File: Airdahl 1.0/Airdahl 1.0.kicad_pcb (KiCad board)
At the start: 2 copper layers, 57.6 x 39.5 mm, 94 parts, among them J1 Conn_01x04, J2 DF40C-34DS-0.4V_58_, J3 DF40C-34DS-0.4V_58_, J4 USB_C_Receptacle_USB2.0_16P, J7 CONUFL001-SMD-T, J9 104031-0811, SW1 SW_SPST, SW2 SW_SPST, U1 STM32F446RETx, U2 MCP2200-I-MQ, U4 BNO085, U5 BMP581, U6 RFM95W-915S2, U7 NCP1117-3.3_SOT223, Y1 ABM3B-8.000MHZ-12-D1X-T, Y2 ABS25-32.768KHZ-6-T, Y3 12MHz

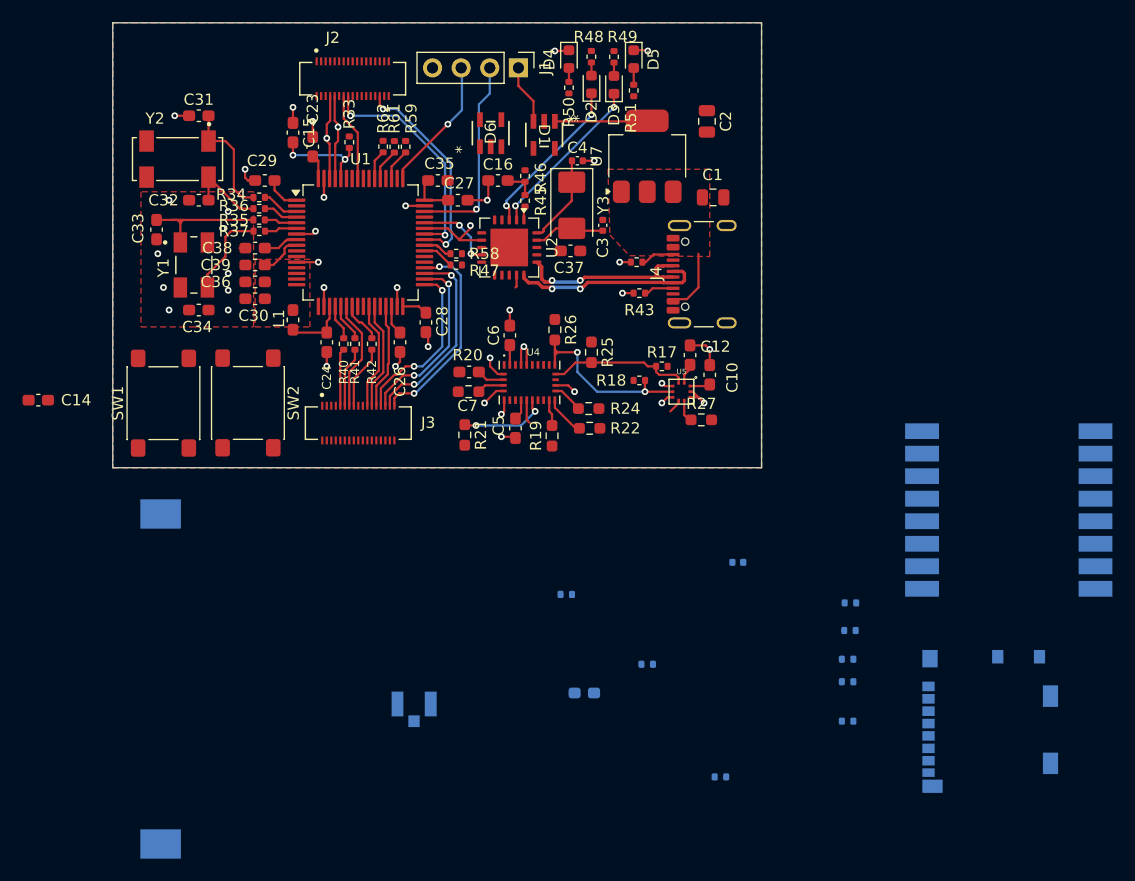
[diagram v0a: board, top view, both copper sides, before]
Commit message: dumping many layout changes
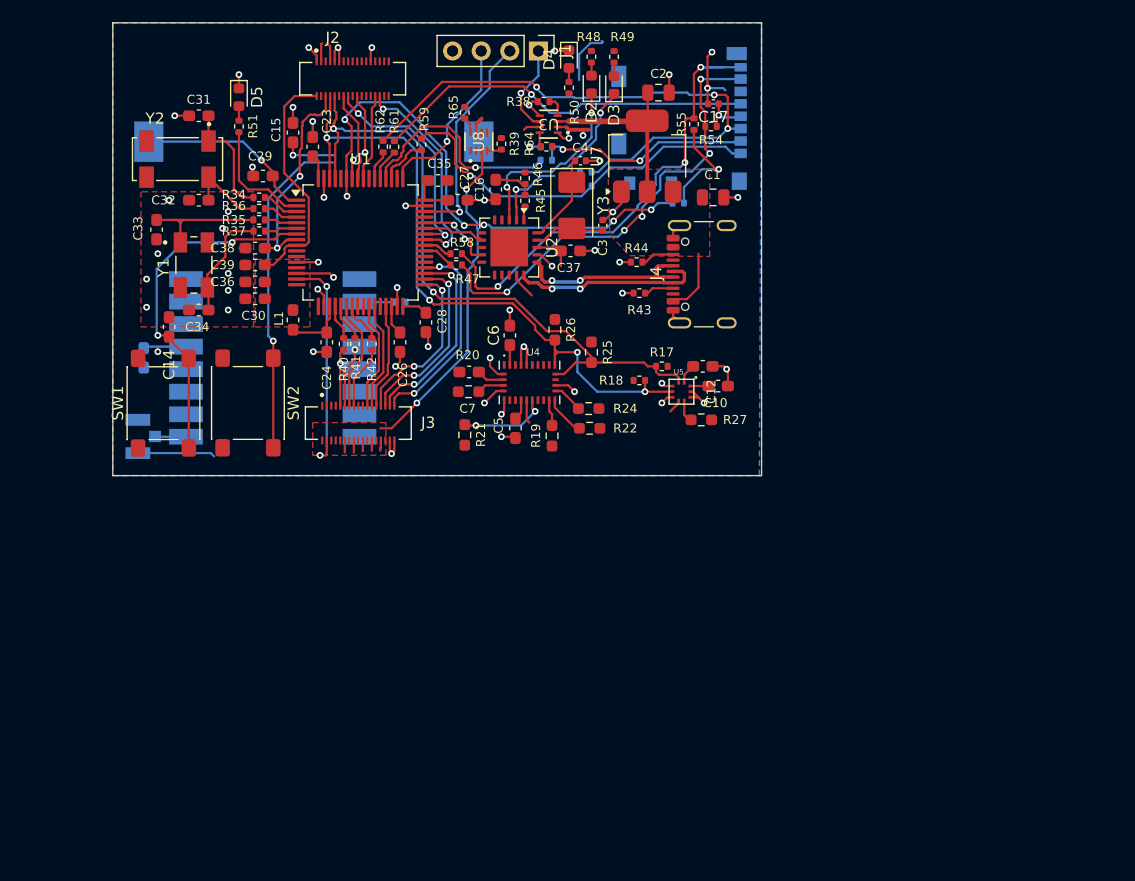
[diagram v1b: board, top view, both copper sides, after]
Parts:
- removed D1, D6: RB496EATR, RB496EATR:DIO_FTZ_ROM
- removed R33: 10K, Resistor_SMD:R_0402_1005Metric
- added R38: 0, Resistor_SMD:R_0402_1005Metric, F.Cu at (160.3, 61.0)
- added R39: 0, Resistor_SMD:R_0402_1005Metric, F.Cu at (156.5, 64.7)
- added R64: 10k, Resistor_SMD:R_0402_1005Metric, F.Cu at (160.5, 65.0)
- added R65: 10k, Resistor_SMD:R_0402_1005Metric, F.Cu at (153.2, 62.0)
- added U3: LM66200DRLR, LM66200DRLR:SOT-5X3_DRL_TEX, F.Cu at (160.7, 63.0)
- added U8: LM66200DRLR, LM66200DRLR:SOT-5X3_DRL_TEX, F.Cu at (154.5, 64.6)
- C17, R54, R55: moved to F.Cu
- moved U6 66.7 mm to (136.2, 83.8)
- moved J9 60.2 mm to (172.3, 62.5), turned to -90 degrees
- moved R60 56.9 mm to (160.5, 66.2), turned to 0 degrees
- moved R53 54.0 mm to (164.0, 67.2)
- moved R54 50.8 mm to (175.1, 63.2), turned to 0 degrees
- moved BT1 49.6 mm to (139.8, 64.6), turned to 0 degrees
- moved R55 49.4 mm to (173.6, 63.0), turned to -90 degrees
- moved C13 49.1 mm to (124.8, 83.8), turned to -90 degrees
- moved R57 48.7 mm to (160.5, 65.0)
- moved R56 45.9 mm to (164.0, 68.5)
- moved R52 41.0 mm to (172.2, 70.0), turned to 0 degrees
- moved C17 40.8 mm to (175.3, 61.2)
- moved D5 35.2 mm to (133.2, 60.6)
- moved R51 35.2 mm to (133.2, 63.2)
- moved J7 34.1 mm to (124.2, 90.7), turned to -90 degrees
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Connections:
- net /PC13 renamed /PAYLOAD_S
- J2 pad 20: /PC5 -> /PAYLOAD_S1
- J2 pad 28: unconnected-(J2-Pad28) -> /PAYLOAD_S2
- J2 pad 3: unconnected-(J2-Pad3) -> +3V3
- J2 pad 7: +3V3_REG -> +3V3
- J3 pad 16: unconnected-(J3-Pad16) -> +3V3_REG
- J3 pad 20: unconnected-(J3-Pad20) -> +3V3_REG
- J3 pad 24: unconnected-(J3-Pad24) -> +3V3_REG
- J3 pad 28: unconnected-(J3-Pad28) -> +3V3_REG
- U1 pad 56: /PB4 -> /PAYLOAD_S2
- U1 pad 58: /PB6 -> /PAYLOAD_S1
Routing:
- net /SDIO_CMD: track 0.00 -> 51.4 mm, vias 0 -> 3
- net /CD: track 0.00 -> 47.6 mm, vias 0 -> 6
- net /SDIO_D1: track 0.00 -> 42.5 mm, vias 0 -> 3
- net /SDIO_D0: track 0.00 -> 40.7 mm, vias 0 -> 5
- net /SCL: track 20.2 -> 59.2 mm, vias 1 -> 2
- net +3V3: track 25.9 -> 64.7 mm, vias 0 -> 5
- net /SDA: track 24.3 -> 59.4 mm, vias 3 -> 4
- net +3V3_REG: track 0.00 -> 34.8 mm, vias 0 -> 2
- net GND: track 50.2 -> 84.9 mm, vias 38 -> 51
- net /SDIO_D2: track 0.00 -> 34.2 mm, vias 0 -> 1
- net /SDIO_CLK: track 0.00 -> 34.1 mm, vias 0 -> 1
- net /NRST: track 1.78 -> 31.3 mm, vias 1 -> 2
- net /BOOT0: track 9.10 -> 34.4 mm
- net Net-(U1-PC11): track 0.00 -> 19.7 mm, vias 0 -> 1
- net /SDIO_D3: track 0.00 -> 19.2 mm, vias 0 -> 2
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- added copper zone on F.Cu, net +3V3_REG
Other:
- board size 57.6 x 39.5 mm -> 57.6 x 40.2 mm
